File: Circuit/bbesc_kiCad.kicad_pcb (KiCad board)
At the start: 2 copper layers, 110.5 x 82.5 mm, 82 parts, among them J1 CONN_01X02, J10 CONN_01X01, J11 CONN_01X01, J12 CONN_01X01, J13 CONN_01X01, J14 CONN_01X01, J15 CONN_01X02, J16 CONN_01X02, J17 CONN_01X01, J18 CONN_01X01, J19 CONN_01X01, J2 CONN_01X06, J3 CONN_01X06, J4 CONN_01X06, J5 CONN_01X02, J6 CONN_01X02, J7 CONN_01X01, J8 CONN_01X01, J9 RJ45, Q1 Q_NMOS_GDS, Q2 Q_NMOS_GDS, Q3 Q_NMOS_GDS, Q4 Q_NMOS_GDS, Q5 Q_NMOS_GDS, Q6 Q_NMOS_GDS, U1 teensy_3-2, U2 IR2101, U3 IR2101, U4 IR2101, U5 LM324N, U6 LM7805

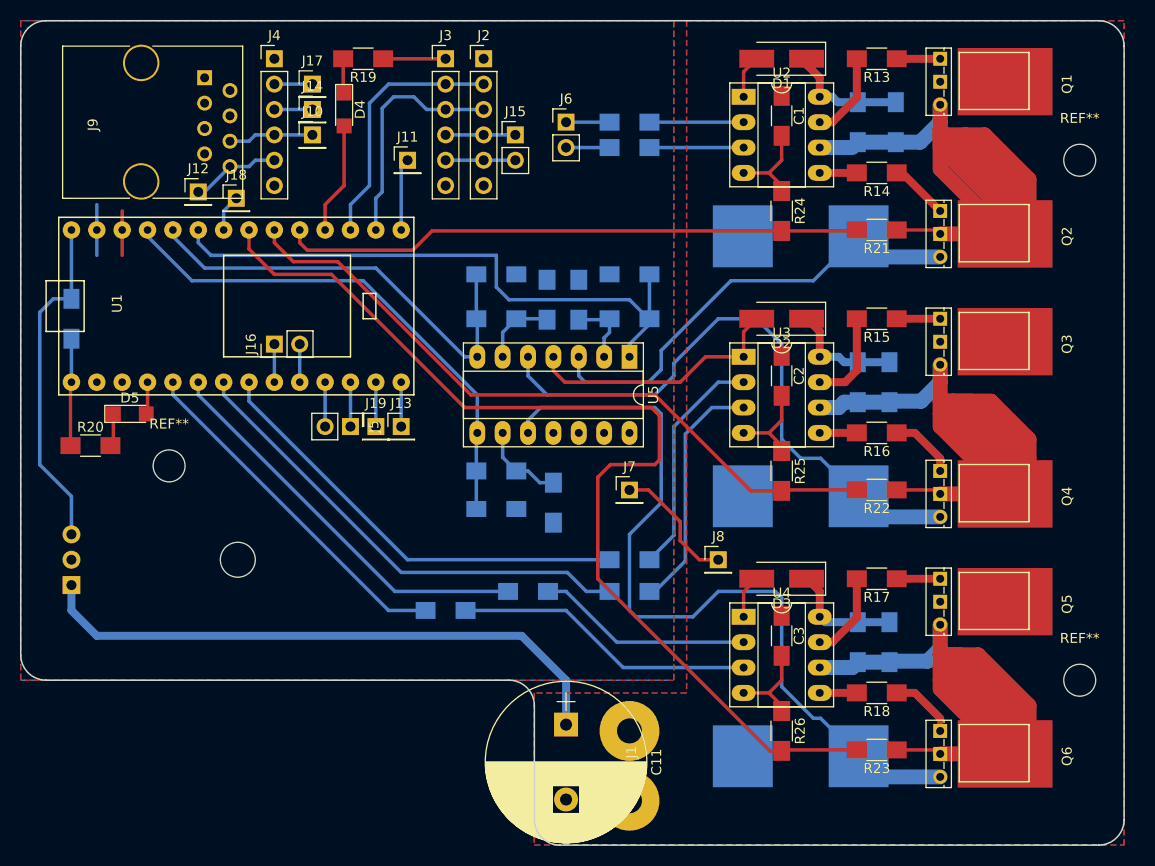
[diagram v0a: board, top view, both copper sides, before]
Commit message: circuit for fab, foc bones
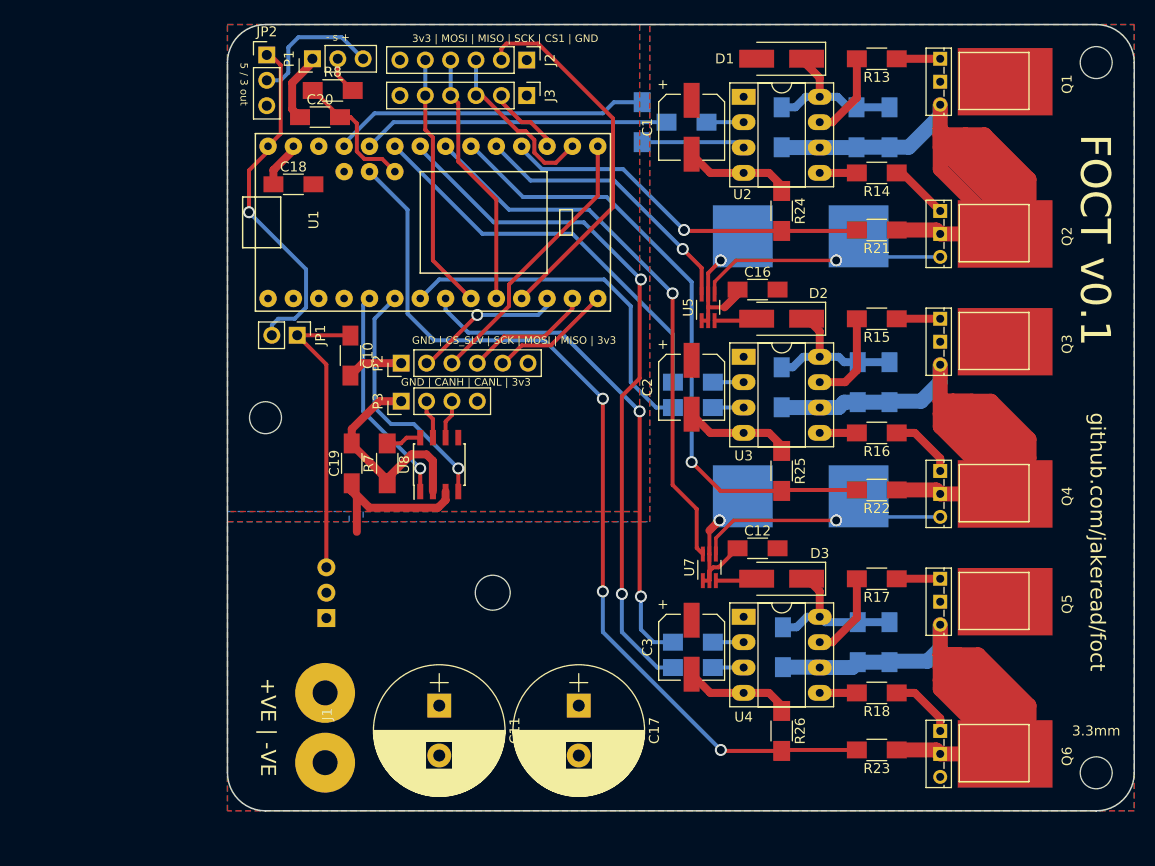
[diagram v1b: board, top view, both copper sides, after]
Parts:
- removed D4, D5: LED, LEDs:LED_1206
- removed J10, J11, J12, J13, J14, J17, J18, J19, J7, J8: CONN_01X01, Pin_Headers:Pin_Header_Straight_1x01_Pitch2.54mm
- removed J15, J16, J5, J6: CONN_01X02, Pin_Headers:Pin_Header_Straight_1x02_Pitch2.54mm
- removed J4: CONN_01X06, Pin_Headers:Pin_Header_Straight_1x06_Pitch2.54mm
- removed J9: RJ45, Connectors:RJ45_8
- removed R10: .001, R_SHUNT_3920:R_2816_HandSoldering
- removed R11, R12, R29: 470k, Resistors_SMD:R_1206_HandSoldering
- removed R19, R20: 4K7, Resistors_SMD:R_1206_HandSoldering
- removed R27: 12k, Resistors_SMD:R_1206_HandSoldering
- removed REF** (x3): MountingHole_3.2mm_M3, Mounting_Holes:MountingHole_3.2mm_M3
- added 3.3mm: MountingHole_3.2mm_M3, Mounting_Holes:MountingHole_3.2mm_M3, F.Cu at (164.2, 144.5)
- added ?: MountingHole_3.2mm_M3, Mounting_Holes:MountingHole_3.2mm_M3, F.Cu at (164.2, 73.4)
- added ?: MountingHole_3.2mm_M3, Mounting_Holes:MountingHole_3.2mm_M3, F.Cu at (81.0, 109.0)
- added C15: 10uF, Capacitors_SMD:C_1206_HandSoldering, B.Cu at (132.8, 132.0)
- added C16: 0.1uF, Capacitors_SMD:C_1206_HandSoldering, F.Cu at (130.3, 96.1)
- added C17: 2000uF, Capacitors_ThroughHole:CP_Radial_D13.0mm_P5.00mm, F.Cu at (112.4, 137.8)
- added C18: 10uF, Capacitors_SMD:C_1206_HandSoldering, F.Cu at (83.8, 85.6)
- added C19: 10uF, Capacitors_SMD:C_1206_HandSoldering, F.Cu at (89.7, 113.5)
- added C20: 10uF, Capacitors_SMD:C_1206_HandSoldering, F.Cu at (86.5, 78.9)
- added JP1: JUMPER, Pin_Headers:Pin_Header_Straight_1x02_Pitch2.54mm, F.Cu at (84.2, 100.7)
- added JP2: JUMPER3, Pin_Headers:Pin_Header_Straight_1x03_Pitch2.54mm, F.Cu at (81.2, 72.6)
- added P1: CONN_01X03, Pin_Headers:Pin_Header_Straight_1x03_Pitch2.54mm, F.Cu at (85.7, 73.0)
- added P2: CONN_01X06, Pin_Headers:Pin_Header_Straight_1x06_Pitch2.54mm, F.Cu at (94.6, 103.5)
- added P3: CONN_01X04, Pin_Headers:Pin_Header_Straight_1x04_Pitch2.54mm, F.Cu at (94.6, 107.3)
- added U7: INA21x, TO_SOT_Packages_SMD:SOT-363_SC-70-6_Handsoldering, F.Cu at (125.5, 124.0)
- added U8: TJA1051T-SN65HVD230D, Housings_SOIC:SOIC-8_3.9x4.9mm_Pitch1.27mm, F.Cu at (98.4, 113.7)
- C1, C2, C3: value 1uF -> 56uF; footprint Capacitors_SMD:C_1206_HandSoldering -> Capacitors_SMD:CP_Elec_6.3x7.7
- C10: moved to F.Cu
- C11: footprint Capacitors_THT:CP_Radial_D16.0mm_P7.50mm -> Capacitors_ThroughHole:CP_Radial_D13.0mm_P5.00mm
- C12: value 100pF -> 0.1uF; moved to F.Cu
- C13, C14: value 100pF -> 10uF
- Q2: footprint TO-251_IPAK_Vertical -> TO-251_IPAK_Slammed:TO-251_IPAK_Vertical
- R1, R2, R3, R4, R5, R6: value 470R -> 220R
- R13, R14, R15, R16, R17, R18: value 47R -> 4R7
- R7: value 12k -> 10K; moved to F.Cu
- R8: value 12k -> 47R; moved to F.Cu
- U5: value LM324N -> INA21x; footprint Housings_DIP:DIP-14_W7.62mm_Socket_LongPads -> TO_SOT_Packages_SMD:SOT-363_SC-70-6_Handsoldering
- moved R8 46.8 mm to (87.8, 76.2), turned to 0 degrees
- moved C12 37.9 mm to (130.3, 122.0)
- moved C14 31.1 mm to (132.7, 105.9), turned to 90 degrees
- moved J1 30.7 mm to (87.0, 143.5)
- moved C13 29.9 mm to (143.5, 79.9), turned to 90 degrees
- moved C10 28.2 mm to (89.5, 102.7)
- moved U6 25.7 mm to (87.1, 129.0)
- moved R6 25.4 mm to (123.8, 134.0)
- moved R7 25.2 mm to (93.2, 113.5)
- moved U1 21.4 mm to (96.5, 89.4)
- moved R4 19.5 mm to (123.8, 108.0)
- moved R3 18.9 mm to (123.8, 105.4)
- moved R5 17.3 mm to (123.8, 131.4)
- moved C11 12.8 mm to (98.4, 137.8)
- moved U5 9.30 mm to (125.3, 97.9), turned to 90 degrees
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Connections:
- net LO_B renamed LO_V
- net PHASE_C renamed PHASE_W
- net V_SENS_B renamed V_SENS_V
- C12 pad 1: A_SENS_B -> GND
- C12 pad 2: GND -> VCC
- C13 pad 1: A_SENS_A -> PHASE_U
- C13 pad 2: GND -> Net-(C13-Pad2)
- C14 pad 1: A_SENS_C -> PHASE_V
- C14 pad 2: GND -> Net-(C14-Pad2)
- C4 pad 1: PHASE_A -> PHASE_U
- C4 pad 2: Net-(C4-Pad2) -> Net-(C13-Pad2)
- C5 pad 1: PHASE_A -> PHASE_U
- C5 pad 2: Net-(C4-Pad2) -> Net-(C13-Pad2)
- C6 pad 1: PHASE_B -> PHASE_V
- C6 pad 2: Net-(C6-Pad2) -> Net-(C14-Pad2)
- C7 pad 1: PHASE_B -> PHASE_V
- C7 pad 2: Net-(C6-Pad2) -> Net-(C14-Pad2)
- D1 pad 1: Net-(C4-Pad2) -> Net-(C13-Pad2)
- D2 pad 1: Net-(C6-Pad2) -> Net-(C14-Pad2)
- J2 pad 4: Net-(J15-Pad1) -> MISO2
- J2 pad 5: Net-(J15-Pad2) -> MOSI2
- J3 pad 2: CS2 -> CS1
- J3 pad 4: Net-(J15-Pad1) -> MISO2
- J3 pad 5: Net-(J15-Pad2) -> MOSI2
- Q1 pad 3: PHASE_A -> PHASE_U
- Q2 pad 2: PHASE_A -> PHASE_U
- Q3 pad 3: PHASE_B -> PHASE_V
- Q4 pad 2: PHASE_B -> PHASE_V
- Q6 pad 3: Net-(Q6-Pad3) -> GND
- R1 pad 2: HI_A -> HI_U
- R2 pad 2: LO_A -> LO_U
- R21 pad 1: PHASE_A -> PHASE_U
- R21 pad 2: V_SENS_A -> V_SENS_U
- R22 pad 1: PHASE_B -> PHASE_V
- R23 pad 2: V_SENS_C -> V_SENS_W
- R24 pad 2: V_SENS_A -> V_SENS_U
- R26 pad 2: V_SENS_C -> V_SENS_W
- R3 pad 2: HI_B -> HI_V
- R5 pad 2: HI_C -> HI_W
- R6 pad 2: LO_C -> LO_W
- R7 pad 1: Net-(R11-Pad2) -> GND
- R7 pad 2: GND -> Net-(R7-Pad2)
- R8 pad 1: Net-(R12-Pad2) -> Net-(C20-Pad2)
- R8 pad 2: GND -> Net-(P1-Pad2)
- U1 pad 10: Net-(J5-Pad1) -> CS0
- U1 pad 15: CS2 -> CS1
- U1 pad 16: Net-(D4-Pad2) -> V_SENS_U
- U1 pad 17: V_SENS_A -> A_SENS_U
- U1 pad 19: V_SENS_C -> A_SENS_V
- U1 pad 20: CS1 -> LO_W
- U1 pad 21: A_SENS_A -> HI_V
- U1 pad 22: A_SENS_B -> HI_U
- U1 pad 23: A_SENS_C -> LO_U
- U1 pad 26: Net-(C10-Pad1) -> 5v
- U1 pad 3: LO_C -> CANTX
- U1 pad 4: HI_C -> CANRX
- U1 pad 6: HI_B -> HI_W
- U1 pad 9: Net-(J5-Pad2) -> CS2
- U2 pad 6: PHASE_A -> PHASE_U
- U2 pad 8: Net-(C4-Pad2) -> Net-(C13-Pad2)
- U3 pad 6: PHASE_B -> PHASE_V
- U3 pad 8: Net-(C6-Pad2) -> Net-(C14-Pad2)
- U5 pad 1: A_SENS_A -> GND
- U5 pad 2: Net-(R11-Pad2) -> GND
- U5 pad 3: Net-(Q2-Pad3) -> VCC
- U5 pad 4: VCC -> Net-(Q2-Pad3)
- U5 pad 5: Net-(Q4-Pad3) -> GND
- U5 pad 6: Net-(R27-Pad1) -> A_SENS_U
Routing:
- net PHASE_U: track 0.00 -> 116.5 mm
- net PHASE_A: track 113.0 -> 0.00 mm
- net V_SENS_C: track 104.5 -> 0.00 mm
- net PHASE_V: track 0.00 -> 99.6 mm
- net PHASE_B: track 95.7 -> 0.00 mm
- net V_SENS_W: track 0.00 -> 92.8 mm, vias 0 -> 3
- net Net-(Q6-Pad3): track 82.5 -> 0.00 mm
- net LO_W: track 0.00 -> 70.6 mm, vias 0 -> 2
- net VCC: track 94.4 -> 25.8 mm
- net A_SENS_A: track 61.1 -> 0.00 mm
- net V_SENS_A: track 58.2 -> 0.00 mm
- net A_SENS_V: track 0.00 -> 56.7 mm, vias 0 -> 1
- net A_SENS_C: track 52.5 -> 0.00 mm
- net HI_W: track 0.00 -> 50.4 mm, vias 0 -> 2
- net HI_B: track 44.6 -> 0.00 mm
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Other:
- board size 110.5 x 82.5 mm -> 90.8 x 78.7 mm
- net class Default: clearance 0.8 -> 0.15; trace_width 0.35 -> 0.4; via_dia 1 -> 1.2
- net class Drive: clearance 0.8 -> 0.2; via_dia 1 -> 1.2
- net class Phase: clearance 0.8 -> 0.2; via_dia 1 -> 1.2
- net class Phase Measurement: clearance 0.8 -> 0.2; via_dia 1 -> 1.2
- rule trace_clearance: 0.8 -> 0.15
- board text added: "+VE | -VE"
- board text added: "- s +"
- board text added: "3v3 | MOSI | MISO | SCK | CS1 | GND"
- board text added: "5 / 3 out"
- board text added: "FOCT v0.1"
- board text added: "GND | CANH | CANL | 3v3"
- board text added: "GND | CS_SLV | SCK | MOSI | MISO | 3v3"
- board text added: "github.com/jakeread/foct"
